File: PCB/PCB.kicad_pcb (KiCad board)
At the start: 2 copper layers, 75 x 75 mm, 14 parts

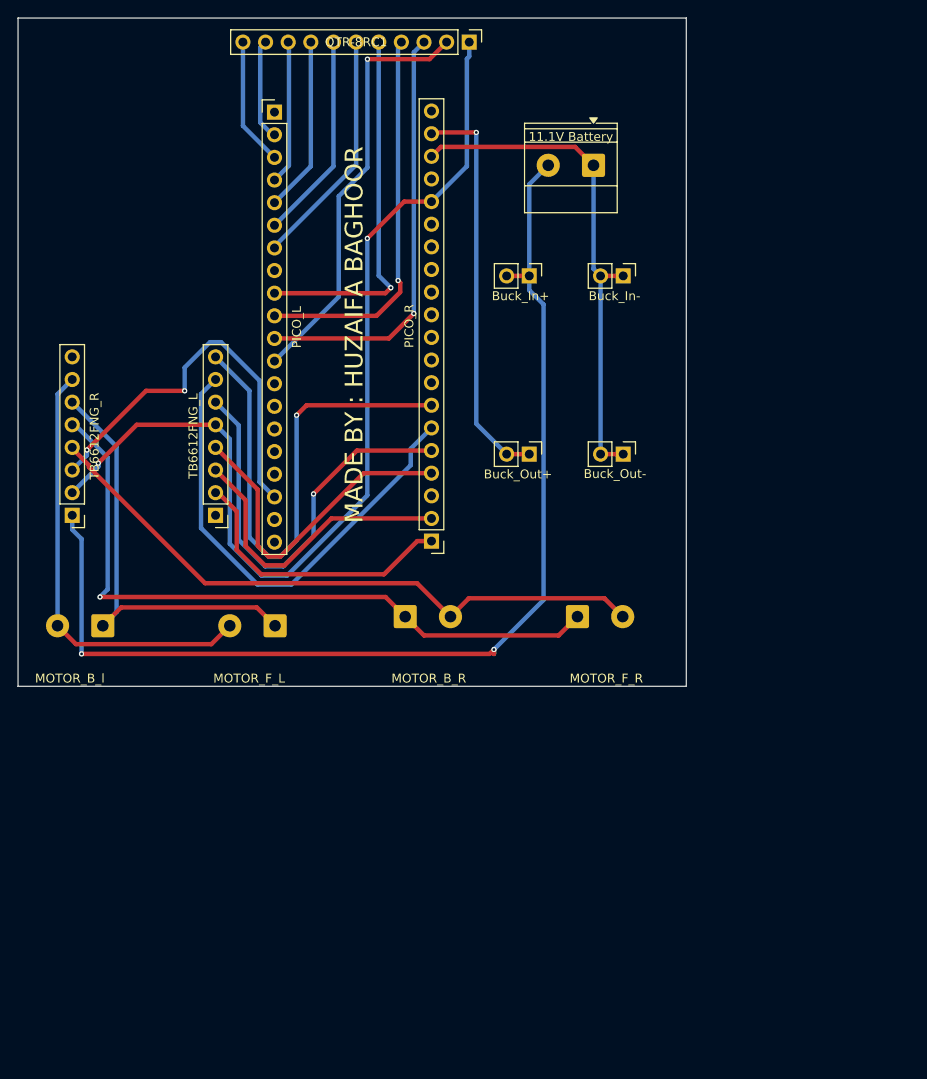
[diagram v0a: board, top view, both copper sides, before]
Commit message: pdf
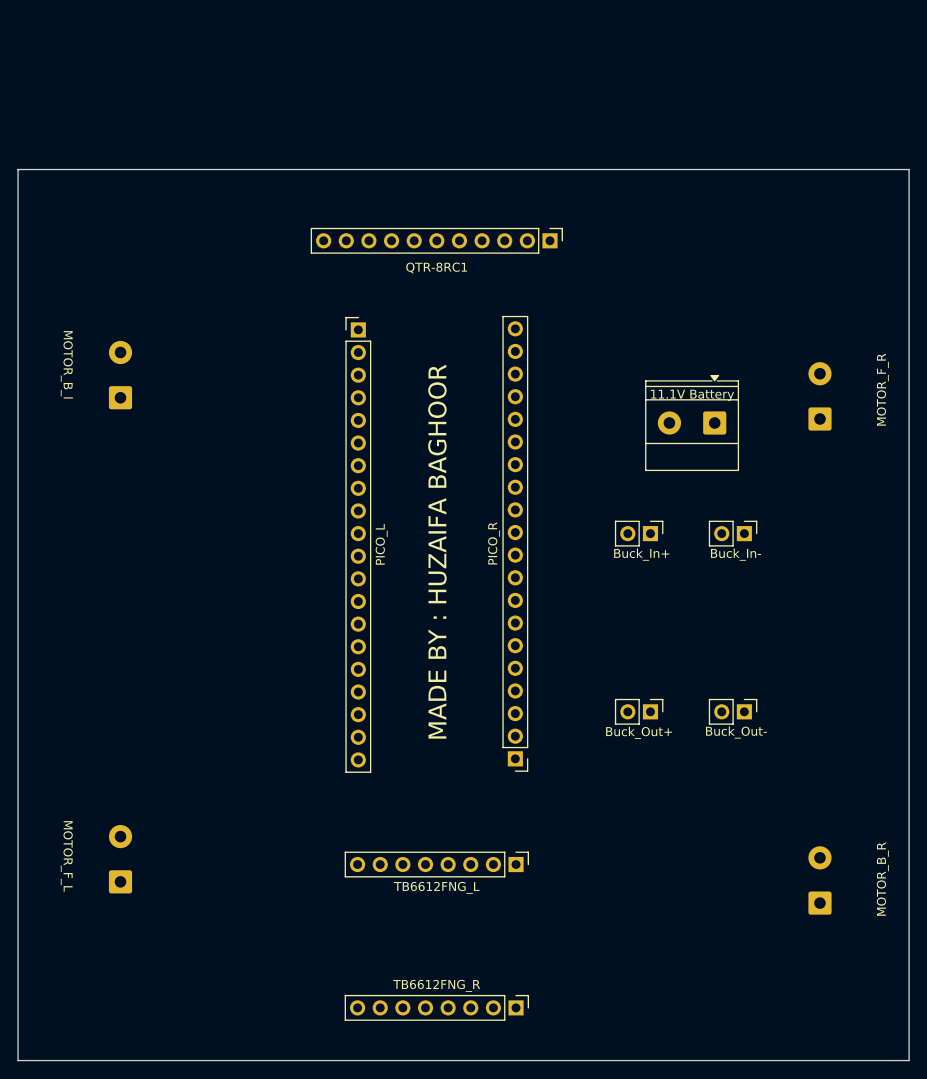
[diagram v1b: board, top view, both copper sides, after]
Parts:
- moved TB6612FNGR1 74.4 mm to (55.9, 111.1), turned to -90 degrees
- moved MotorBR1 56.6 mm to (90.0, 99.3), turned to 90 degrees
- moved TB6612FNGL1 51.7 mm to (55.9, 95.0), turned to -90 degrees
- moved MotorFR1 35.1 mm to (90.0, 45.0), turned to 90 degrees
- moved MotorFL1 33.6 mm to (11.5, 96.9), turned to 90 degrees
- moved Buck_OUT+1 32.0 mm to (71.0, 77.9)
- moved Buck_OUT-1 32.0 mm to (81.5, 77.9)
- moved Battery1 32.0 mm to (78.2, 45.4)
- moved Buck_IN+1 32.0 mm to (71.0, 57.9)
- moved Buck_IN-1 32.0 mm to (81.5, 57.9)
- moved PicoL1 26.2 mm to (38.2, 35.0)
- moved PicoR1 26.2 mm to (55.8, 83.1)
- moved MotorBL1 25.7 mm to (11.5, 42.6), turned to 90 degrees
- moved QTR-8RC1 24.1 mm to (59.7, 25.0)
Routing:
- net VCC: track 125.2 -> 0.00 mm, vias 2 -> 0
- net /3V3_OUT: track 111.5 -> 0.00 mm, vias 2 -> 0
- net Net-(MotorBR1-Pin_1): track 77.8 -> 0.00 mm, vias 1 -> 0
- net Net-(MotorBR1-Pin_2): track 71.6 -> 0.00 mm
- net Net-(PicoR1-Pin_7): track 58.4 -> 0.00 mm, vias 1 -> 0
- net GND: track 57.3 -> 0.00 mm
- net Net-(PicoR1-Pin_6): track 54.2 -> 0.00 mm
- net Net-(MotorBL1-Pin_2): track 49.4 -> 0.00 mm
- net Net-(MotorBL1-Pin_1): track 48.8 -> 0.00 mm
- net Net-(PicoL1-Pin_12): track 47.9 -> 0.00 mm, vias 1 -> 0
- net Net-(PicoL1-Pin_11): track 47.7 -> 0.00 mm, vias 1 -> 0
- net Net-(PicoR1-Pin_5): track 47.6 -> 0.00 mm, vias 1 -> 0
- net /BuckOut: track 45.1 -> 0.00 mm, vias 1 -> 0
- net GND18: track 44.4 -> 0.00 mm, vias 2 -> 0
- net Net-(PicoL1-Pin_10): track 43.5 -> 0.00 mm, vias 1 -> 0
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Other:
- board size 75 x 75 mm -> 100 x 100 mm
